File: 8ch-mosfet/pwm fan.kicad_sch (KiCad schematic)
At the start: 4 parts, among them M1 Fan_4pin

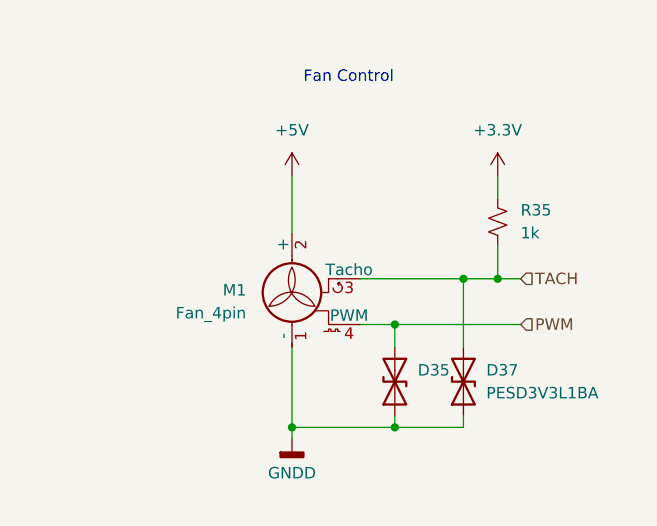
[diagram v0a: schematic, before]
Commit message: more progress on new 8ch board.
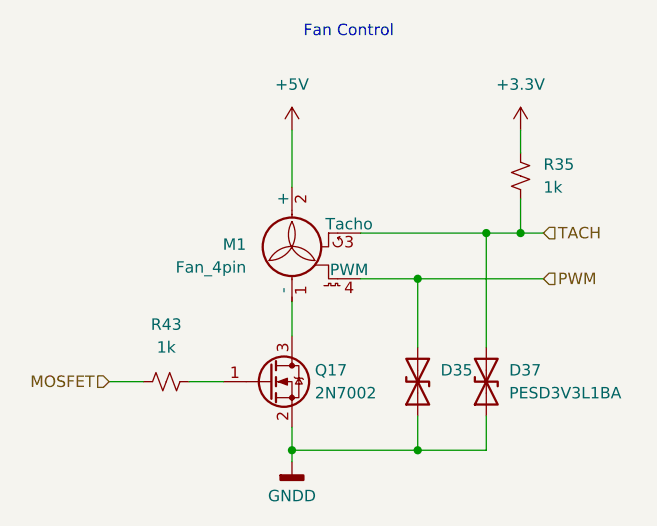
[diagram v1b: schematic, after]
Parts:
- added Q17: 2N7002, Package_TO_SOT_SMD:SOT-23, symbol Transistor_FET:2N7002
- added R43: 1k, Resistor_SMD:R_0805_2012Metric_Pad1.20x1.40mm_HandSolder, symbol Device:R_Small_US
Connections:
- net GNDD: now also Q17.2 (S); no longer M1.1 (-)
- new net: M1.1 (-), Q17.3 (D)
- new net: Q17.1 (G), R43.1
- new net MOSFET: R43.2
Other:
- moved on the sheet: D35, D37, M1, R35
